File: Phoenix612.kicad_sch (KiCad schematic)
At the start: 0 parts

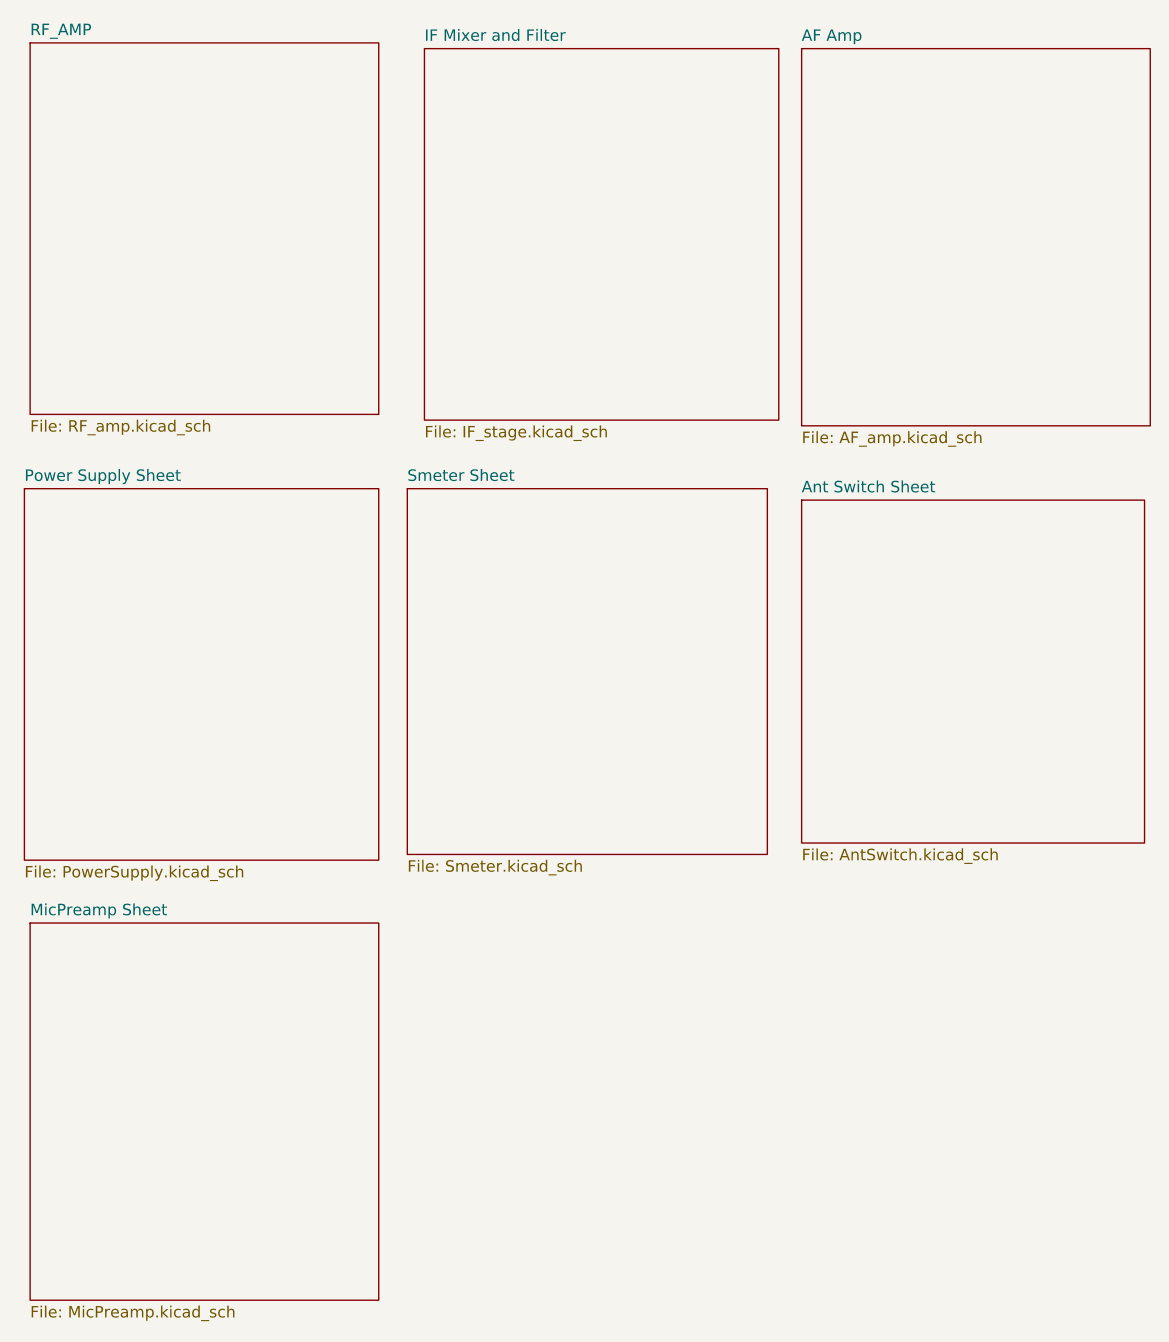
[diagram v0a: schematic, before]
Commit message: Update
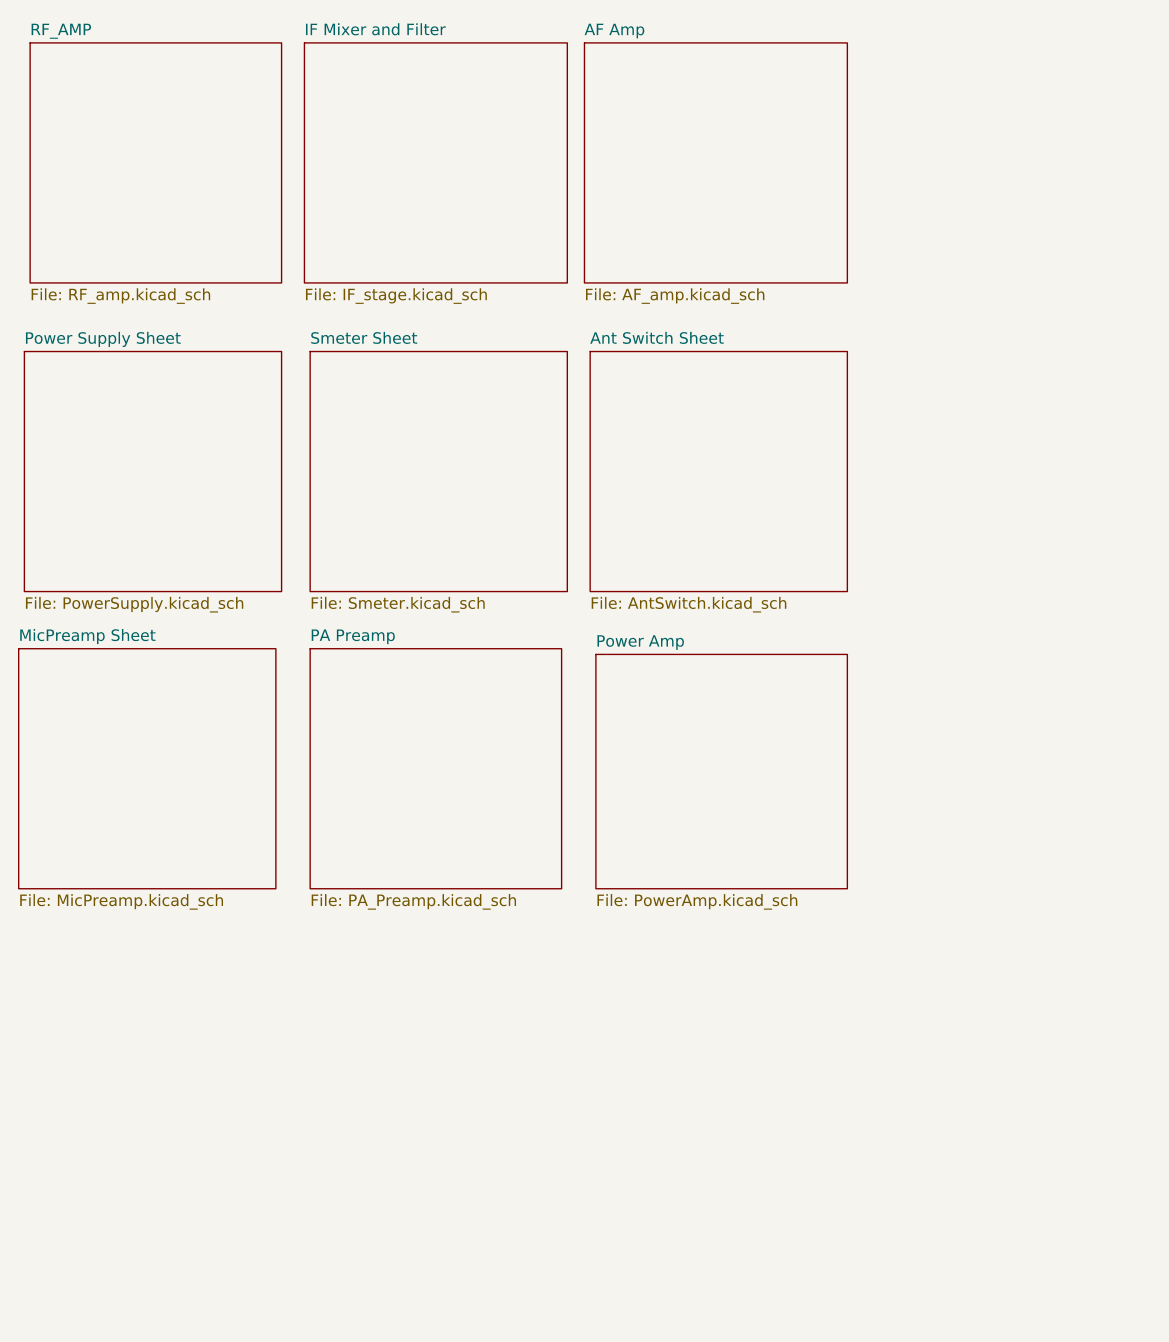
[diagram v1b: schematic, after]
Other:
- added sheet PA Preamp (PA_Preamp.kicad_sch)
- added sheet Power Amp (PowerAmp.kicad_sch)
